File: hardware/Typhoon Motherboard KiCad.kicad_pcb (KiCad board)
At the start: 2 copper layers, 72.9 x 52.1 mm, 61 parts, among them J1 Conn_01x04_Pin, J10 USB_C_Receptacle_USB2.0, J11 Conn_01x02_Pin, J12 Conn_01x02_Pin, J13 Conn_01x02_Pin, J14 Conn_01x02_Pin, J15 Conn_01x02_Pin, J16 Conn_01x02_Pin, J2 Conn_02x03_Odd_Even, J3 Conn_01x04_Pin, U1 ESP32-S3-WROOM-1, U2 SN65HVD233, U4 TPS54331DDA, U7 MCP1825S

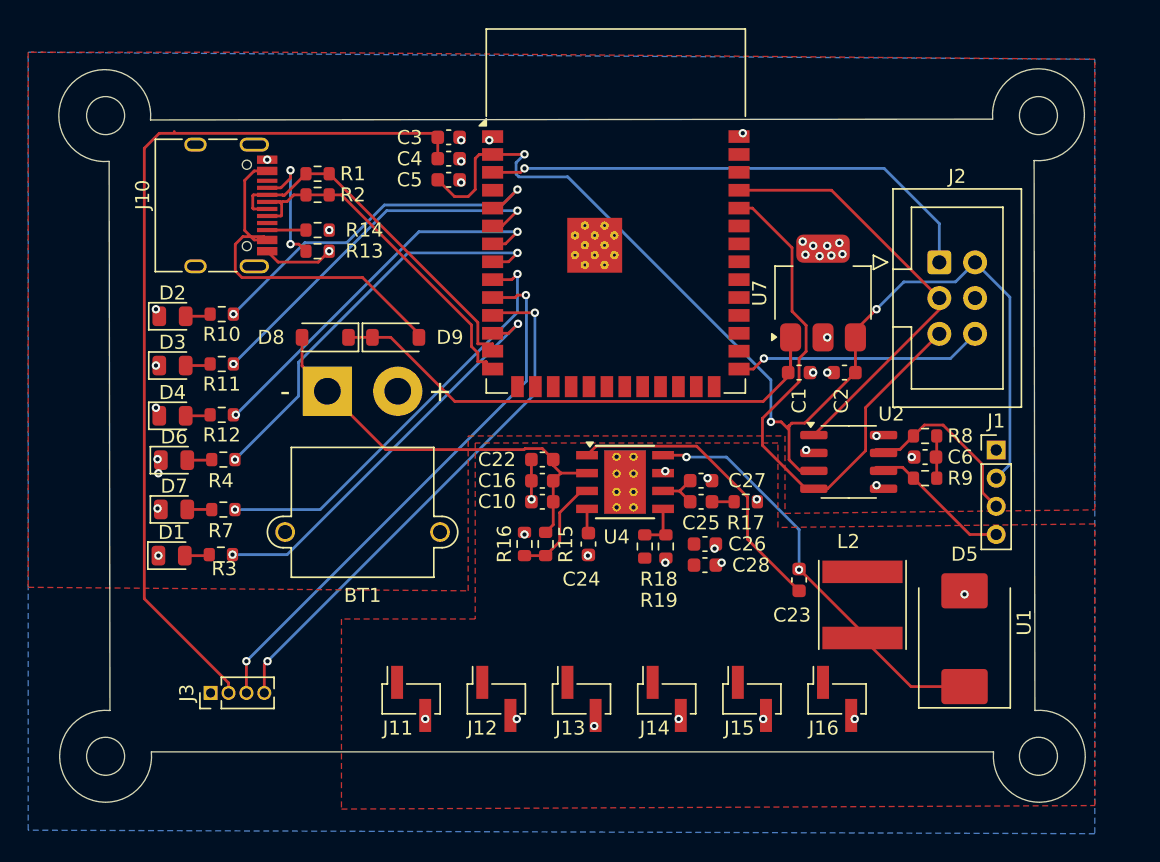
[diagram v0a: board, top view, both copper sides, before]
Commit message: Final Edit
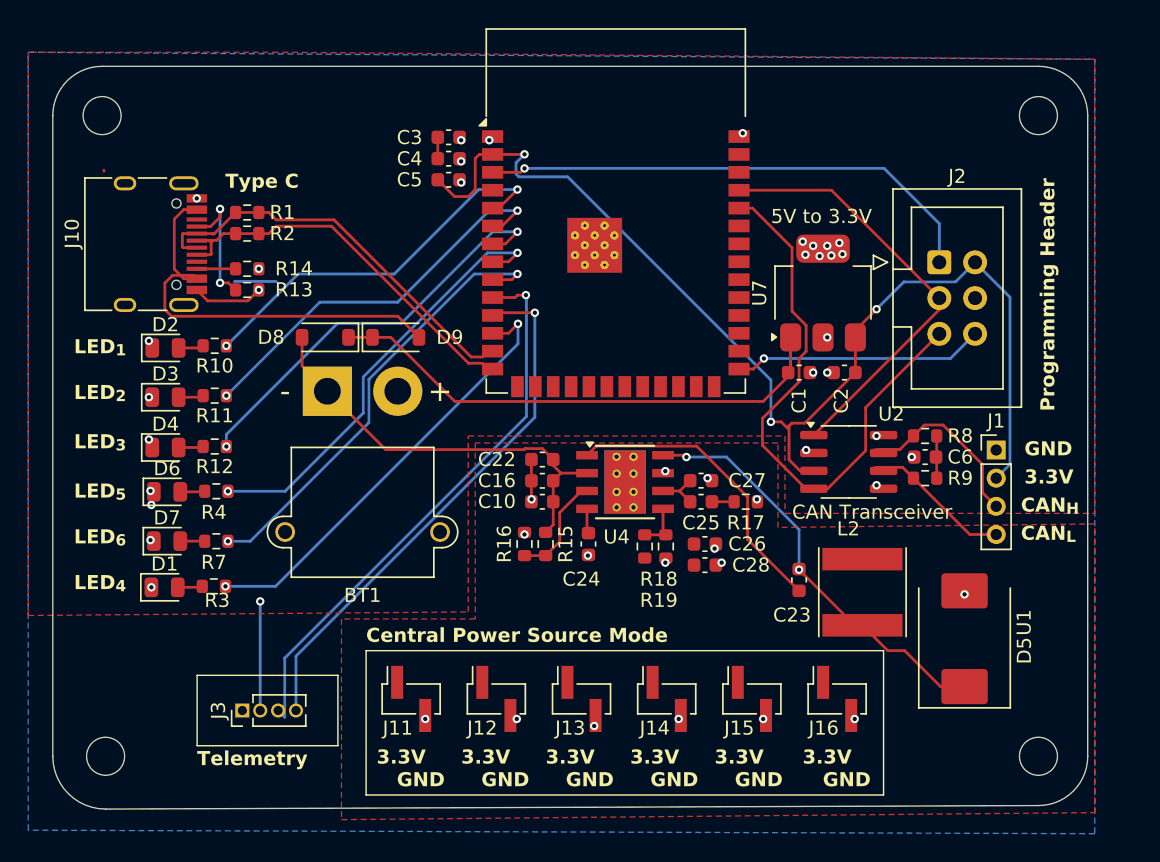
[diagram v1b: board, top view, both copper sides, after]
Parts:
- moved J10 5.71 mm to (107.7, 88.4)
- moved R1 5.71 mm to (115.3, 86.1)
- moved R13 5.71 mm to (115.3, 91.6)
- moved R14 5.71 mm to (115.3, 90.1)
- moved R2 5.71 mm to (115.3, 87.6)
- moved J3 2.57 mm to (115.0, 121.5)
- moved D1 2.30 mm to (109.4, 112.8)
- moved D2 2.30 mm to (109.5, 95.8)
- moved D3 2.30 mm to (109.5, 99.2)
- moved D4 2.30 mm to (109.5, 102.8)
- moved D6 2.30 mm to (109.6, 106.0)
- moved D7 2.30 mm to (109.6, 109.5)
- moved R10 2.30 mm to (113.0, 95.6)
- moved R11 2.30 mm to (113.0, 99.1)
- moved R12 2.30 mm to (113.0, 102.8)
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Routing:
- net +3.3V: track 144.8 -> 90.0 mm, vias 3 -> 4
- net VDC: track 26.9 -> 30.9 mm
- net /D-: track 26.1 -> 29.1 mm
- net /D+: track 25.6 -> 28.6 mm
- net GND: track 8.06 -> 11.0 mm
- net /LED_{4}: track 29.1 -> 31.4 mm
- net /LED_{3}: track 27.5 -> 29.6 mm
- net /LED_{6}: track 30.5 -> 32.2 mm
- net /LED_{5}: track 29.6 -> 31.1 mm
- net /LED_{2}: track 26.9 -> 28.3 mm
- net /LED_{1}: track 26.2 -> 27.6 mm
- net /Mother_{TX}: track 38.9 -> 40.2 mm, vias 2 -> 1
- net /Mother_{RX}: track 38.0 -> 38.4 mm, vias 2 -> 1
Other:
- board size 72.9 x 52.1 mm -> 73.5 x 52.8 mm
- board text added: "3.3V"
- board text added: "3.3V GND"
- board text added: "5V to 3.3V"
- board text added: "CAN Transceiver"
- board text added: "CAN_{H}"
- board text added: "CAN_{L}"
- board text added: "Can be used as central power source"
- board text added: "Central Power Source Mode"
- board text added: "GND"
- board text added: "LED_{1}"
- board text added: "LED_{2}"
- board text added: "LED_{3}"
- board text added: "LED_{4}"
- board text added: "LED_{5}"
- board text added: "LED_{6}"
- board text added: "Programming Header"
- board text added: "Telemetry"
- board text added: "Type C"
- board text added: "Typhoon Motherboard Designed by Jaden Stanshall, Justin Lo"
